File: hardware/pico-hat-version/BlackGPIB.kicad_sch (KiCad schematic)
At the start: 7 parts, among them J1 SD_Card_Module, J2 Raspberry_Pi_Connector

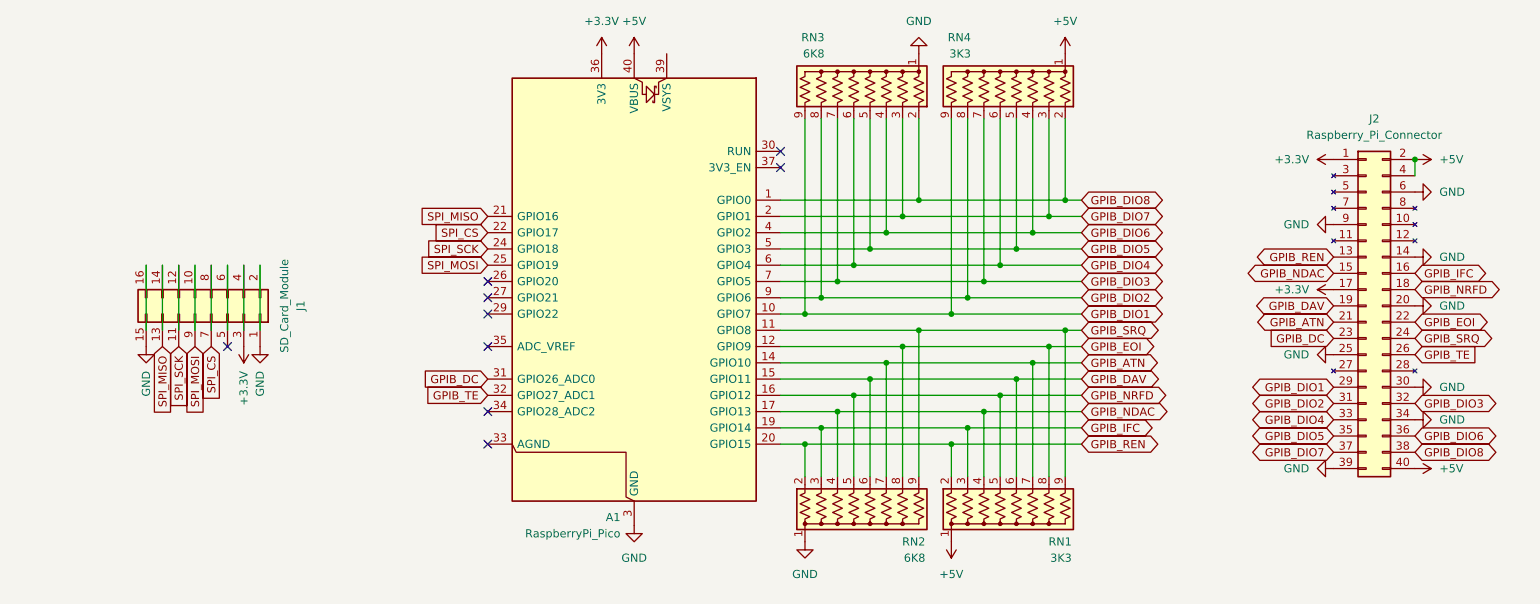
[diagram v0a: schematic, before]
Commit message: pcb
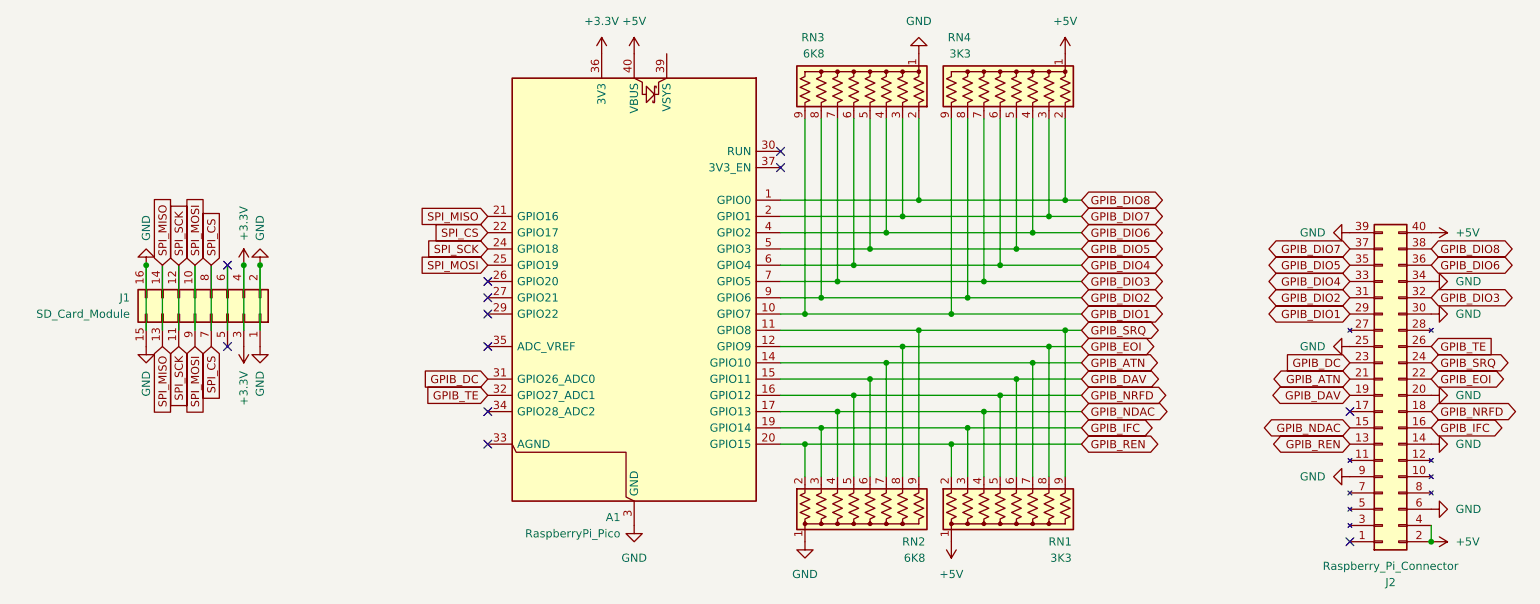
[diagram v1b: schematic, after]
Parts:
- A1: footprint Module:RaspberryPi_Pico_Common_Unspecified -> Module:RaspberryPi_Pico_W_SMD_HandSolder
- J1: footprint (none) -> Connector_PinHeader_2.54mm:PinHeader_2x08_P2.54mm_Vertical_SMD
- J2: footprint (none) -> Connector_PinHeader_2.54mm:PinHeader_2x20_P2.54mm_Vertical_SMD
- RN1, RN4: footprint Resistor_THT:R_Array_SIP9 -> custom:PinHeader_1x09_P2.54mm_Horizontal_Left
- RN2, RN3: footprint Resistor_THT:R_Array_SIP9 -> custom:PinHeader_1x09_P2.54mm_Horizontal_Right
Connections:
- net +3.3V: now also J1.4 (3.3V); no longer J2.1 (3.3V), J2.17 (3.3V)
- net GND: now also J1.16 (GND), J1.2 (GND)
- net SPI_CS: now also J1.8 (CS)
- net SPI_MISO: now also J1.14 (MISO)
- net SPI_MOSI: now also J1.10 (MOSI)
- net SPI_SCK: now also J1.12 (SCK)
- no-connect marks 9 -> 12
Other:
- moved on the sheet: J2
